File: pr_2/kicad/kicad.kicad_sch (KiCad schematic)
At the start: 1 part, among them U1 NUCLEO64-F411RE

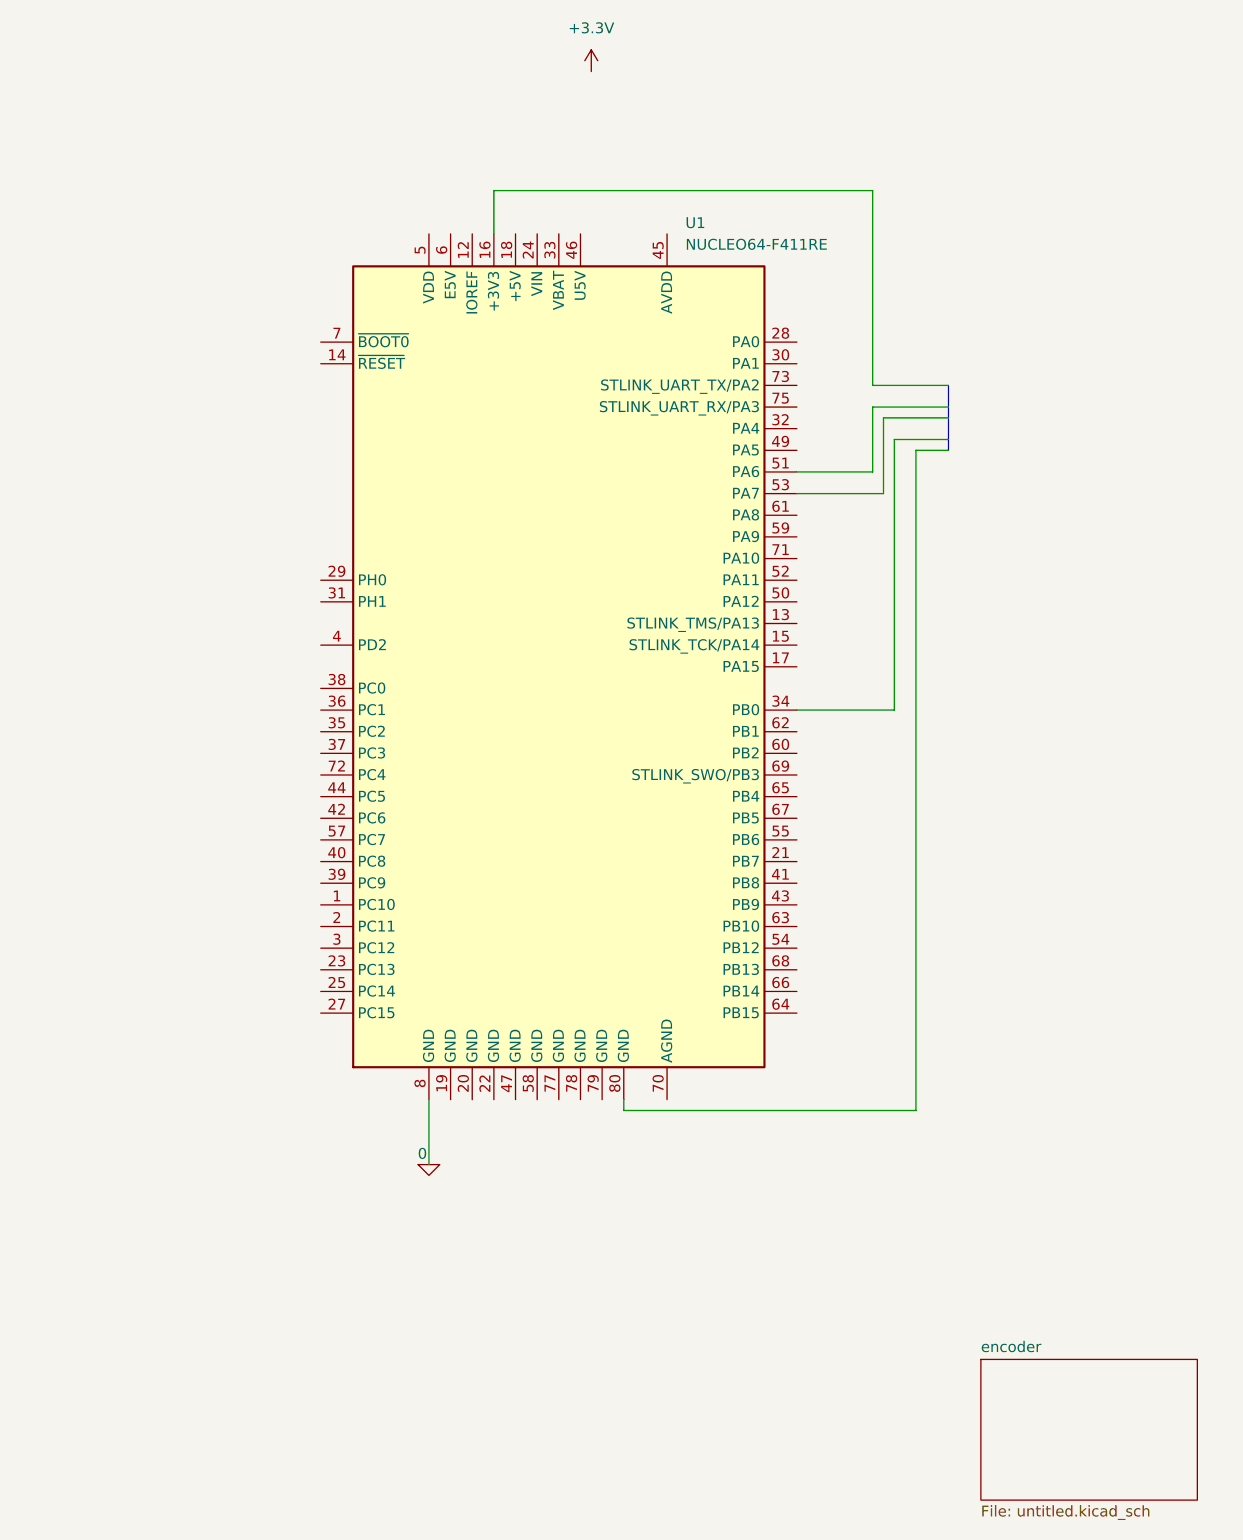
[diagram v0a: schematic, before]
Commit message: feat: added kicad schema
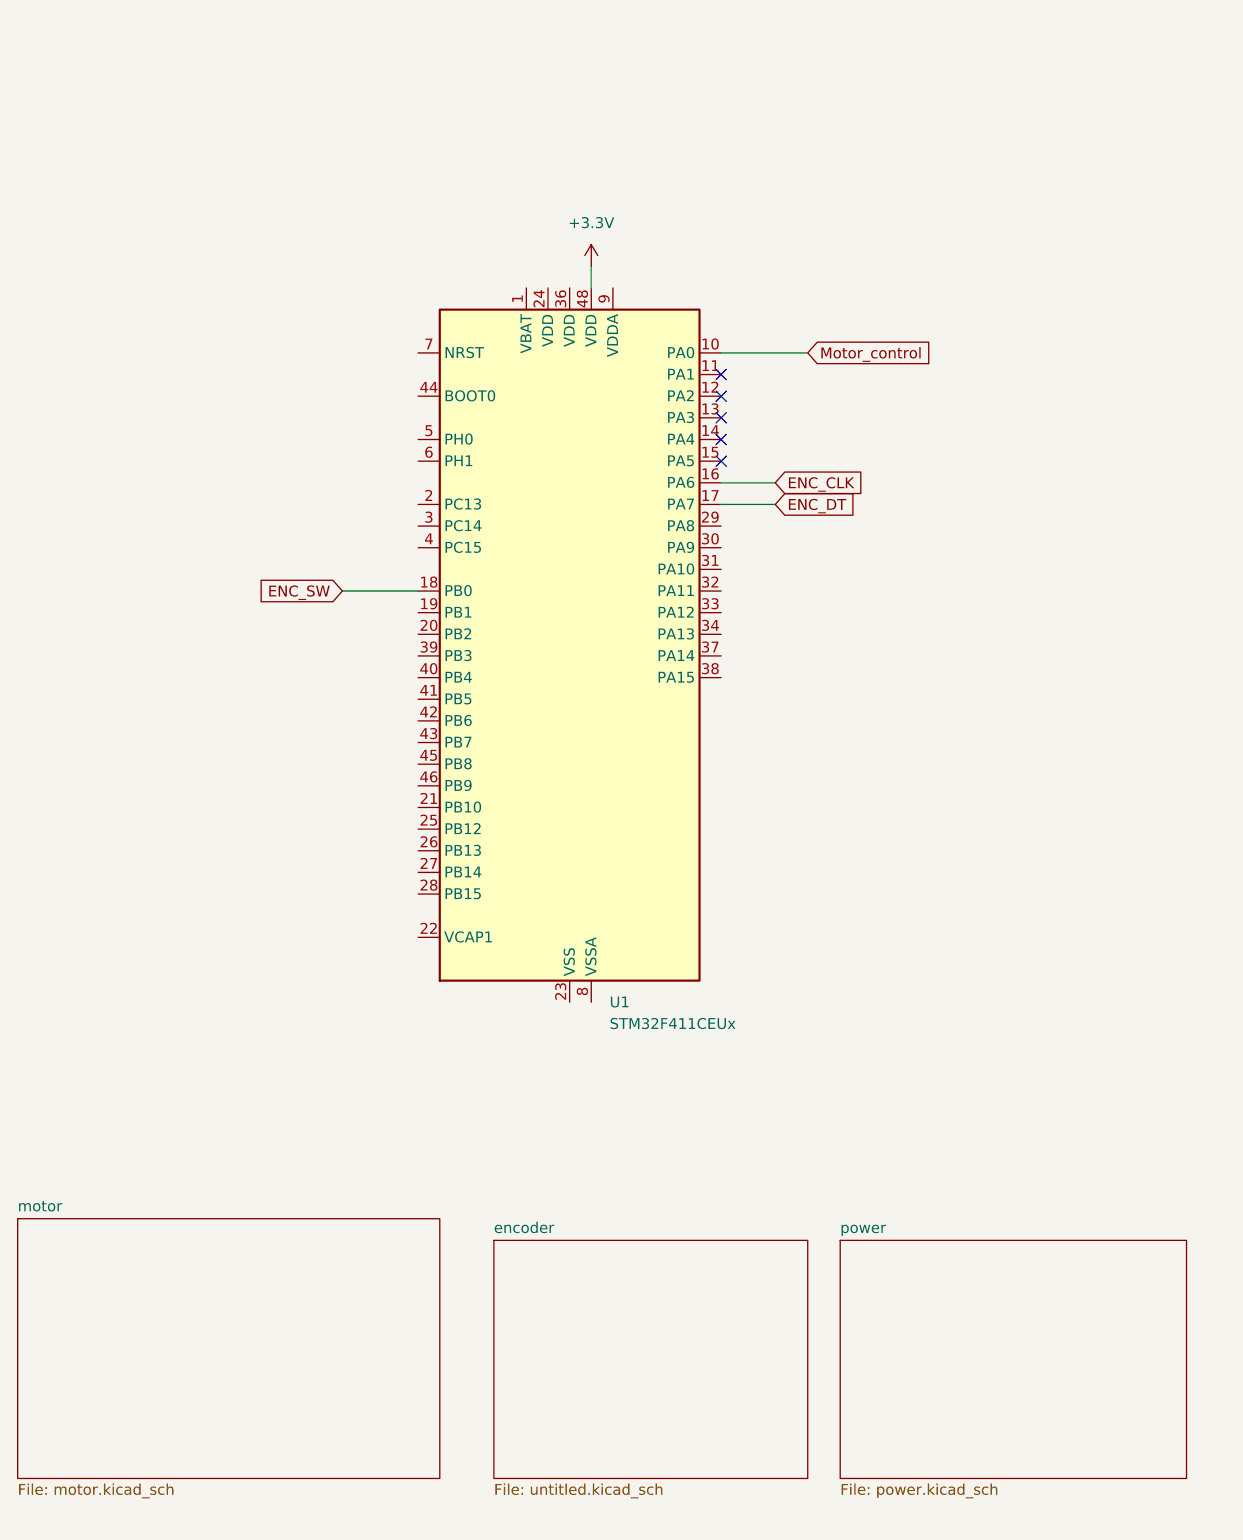
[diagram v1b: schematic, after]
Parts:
- removed U1: NUCLEO64-F411RE, Module:ST_Morpho_Connector_144_STLink, symbol MCU_Module:NUCLEO64-F411RE
- added U1: STM32F411CEUx, Package_DFN_QFN:QFN-48-1EP_7x7mm_P0.5mm_EP5.6x5.6mm, symbol MCU_ST_STM32F4:STM32F411CEUx
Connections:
- net +3.3V: now also U1.48 (VDD)
- new net: U1.23 (VSS), U1.35 (VSS), U1.47 (VSS), U1.49 (VSS)
- new net ENC_CLK: U1.16 (PA6)
- new net ENC_DT: U1.17 (PA7)
- new net ENC_SW: U1.18 (PB0)
- new net Motor_control: U1.10 (PA0)
- no-connect marks 0 -> 5
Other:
- added sheet motor (motor.kicad_sch)
- added sheet power (power.kicad_sch)
